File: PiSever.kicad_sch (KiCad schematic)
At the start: 11 parts, among them J1 USB Power IN, J2 Fan, J3 BMP, J4 RX Ant, J5 TX Ant, J6 USB Power OUT, U1 QFM-RX1-433, U2 AK-FST

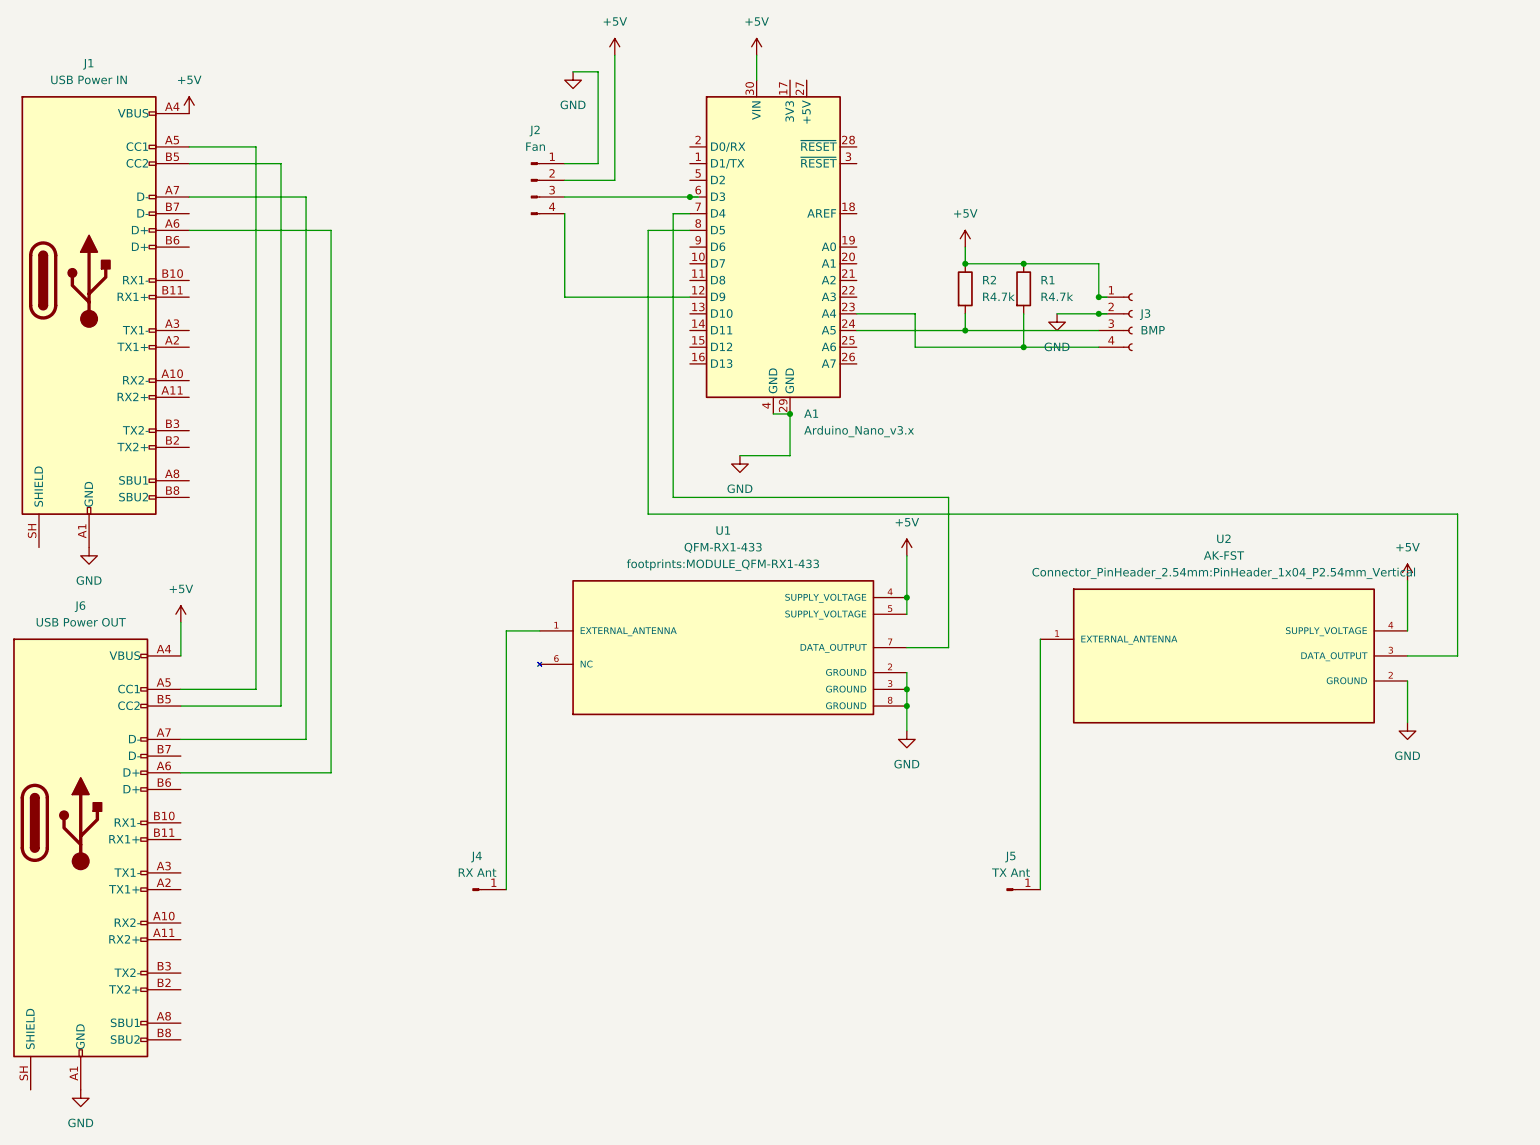
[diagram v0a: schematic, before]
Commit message: Re-route
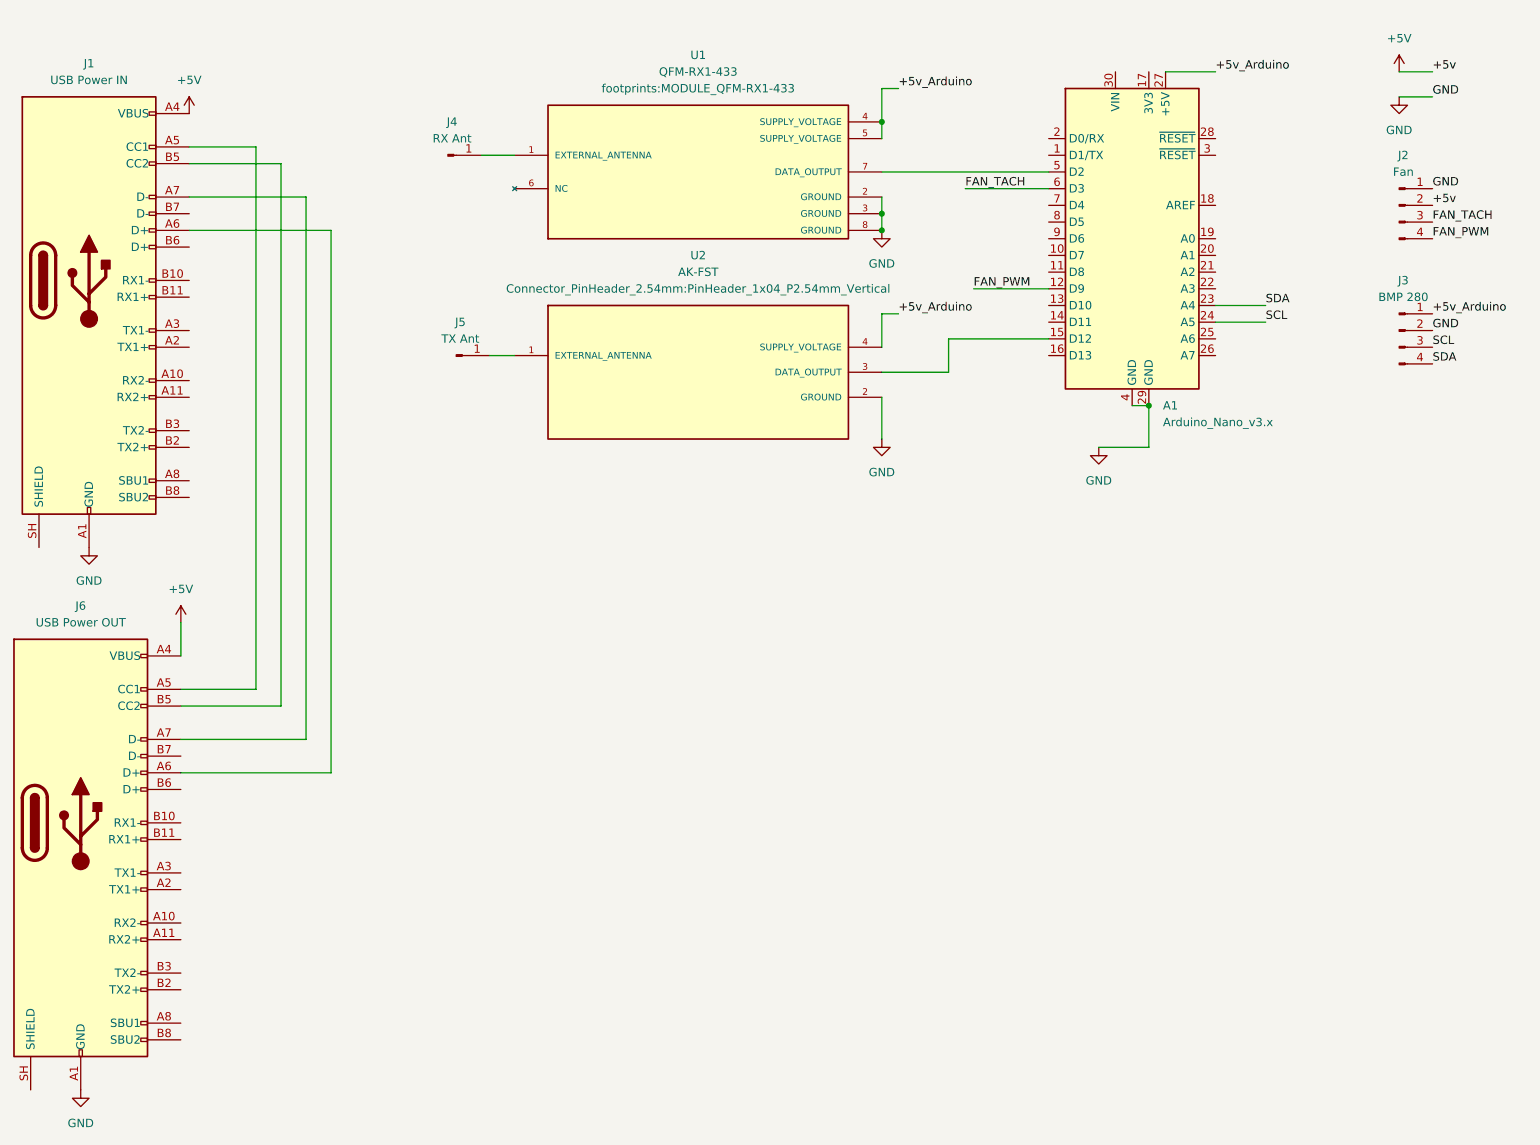
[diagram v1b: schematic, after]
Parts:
- removed J3: BMP, Connector_PinSocket_2.54mm:PinSocket_1x04_P2.54mm_Vertical, symbol Connector:Conn_01x04_Socket
- removed R1, R2: R4.7k, Resistor_THT:R_Axial_DIN0207_L6.3mm_D2.5mm_P7.62mm_Horizontal, symbol Device:R
- added J3: BMP 280, symbol Connector:Conn_01x04_Pin
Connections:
- net +5V: no longer A1.30 (VIN), U1.4 (SUPPLY_VOLTAGE), U1.5 (SUPPLY_VOLTAGE), U2.4 (SUPPLY_VOLTAGE)
- net GND: now also J3.2 (Pin_2)
- net FAN_TACH: now reaches A1.6 (D3), J2.3 (Pin_3)
- net FAN_PWM: now reaches A1.12 (D9), J2.4 (Pin_4)
- net SDA: now reaches A1.23 (A4)
- net SDA: now also J3.4 (Pin_4)
- net SCL: now reaches A1.24 (A5)
- net SCL: now also J3.3 (Pin_3)
- net at A1.15 (D12): now also U2.3 (DATA_OUTPUT)
- net +5v_Arduino: now reaches A1.27 (+5V)
- net +5v_Arduino: now also U1.4 (SUPPLY_VOLTAGE), U1.5 (SUPPLY_VOLTAGE), U2.4 (SUPPLY_VOLTAGE), J3.1 (Pin_1)
- net at A1.5 (D2): now also U1.7 (DATA_OUTPUT)
- net at A1.7 (D4): no longer U1.7 (DATA_OUTPUT)
- net at A1.8 (D5): no longer U2.3 (DATA_OUTPUT)
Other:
- moved on the sheet: A1, J2, J4, J5, U1, U2
